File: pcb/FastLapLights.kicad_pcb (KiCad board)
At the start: 4 copper layers, 27.3 x 40 mm, 17 parts, among them J1 POWER_CON, J2 SWD, J3 PWR, J4 I2C, J5 Conn_02x04_Counter_Clockwise, U1 BD33FC0FP, U2 STM32C011F4Px

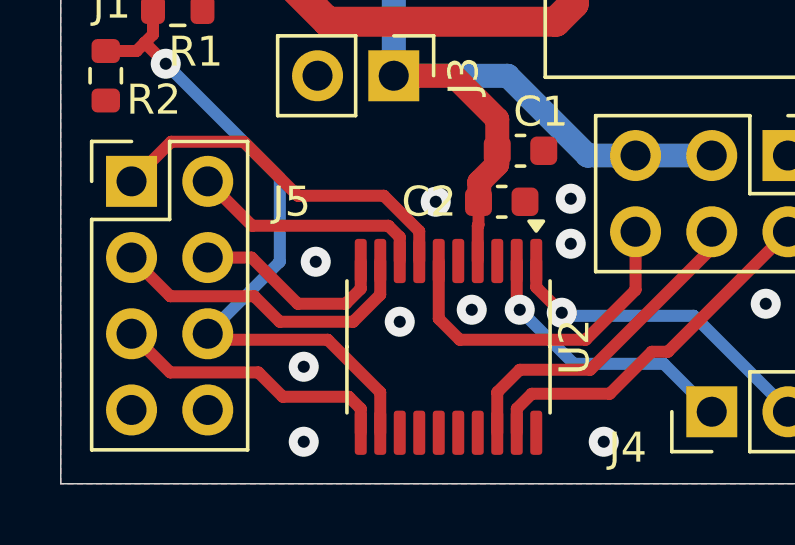
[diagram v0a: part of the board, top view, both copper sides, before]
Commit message: prep firmware
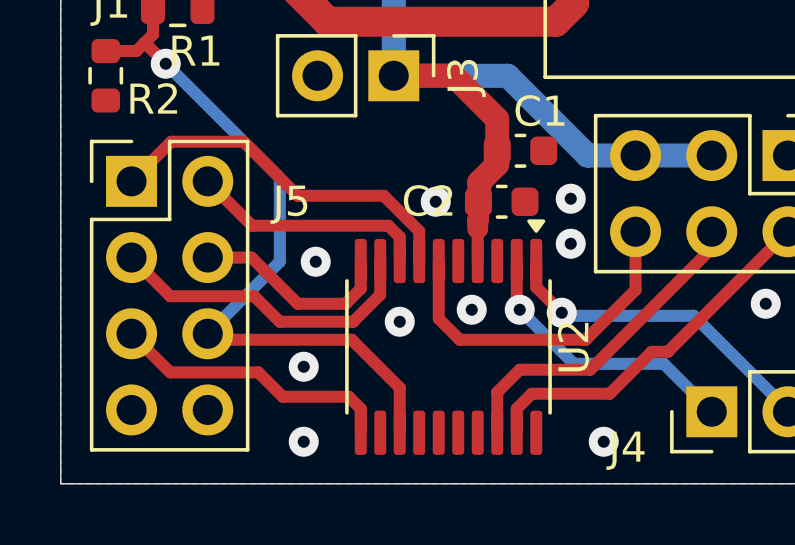
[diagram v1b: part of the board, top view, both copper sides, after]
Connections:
- U2 pad 12: /IO_POWER_RAIL_DATA -> unconnected-(U2-PA5-Pad12)
- U2 pad 13: unconnected-(U2-PA6-Pad13) -> /IO_POWER_RAIL_DATA
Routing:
- net /IO_POWER_RAIL_DATA: track 23.1 -> 23.8 mm
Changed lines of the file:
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@@
 	(net 13 "unconnected-(U2-PA9{slash}PA11-Pad16)")
 	(net 14 "unconnected-(U2-PC15-Pad3)")
-	(net 15 "unconnected-(U2-PA6-Pad13)")
+	(net 15 "unconnected-(U2-PA5-Pad12)")
 	(net 16 "unconnected-(U2-PA10{slash}PA12-Pad17)")
 	(net 17 "VRAIL")
@@
 			(layers "F.Cu" "F.Paste" "F.Mask")
 			(roundrect_rratio 0.25)
-			(net 18 "/IO_POWER_RAIL_DATA")
+			(net 15 "unconnected-(U2-PA5-Pad12)")
 			(pinfunction "PA5")
-			(pintype "bidirectional")
+			(pintype "bidirectional+no_connect")
 		)
 		(pad "13" smd roundrect
@@
 			(layers "F.Cu" "F.Paste" "F.Mask")
 			(roundrect_rratio 0.25)
-			(net 15 "unconnected-(U2-PA6-Pad13)")
+			(net 18 "/IO_POWER_RAIL_DATA")
 			(pinfunction "PA6")
-			(pintype "bidirectional+no_connect")
+			(pintype "bidirectional")
 		)
 		(pad "14" smd roundrect
@@
 		(layer "Cmts.User")
 		(pts
-			(xy 42.5 86.7) (xy 42.5 126.7)
+			(xy 42.5 86.7) (xy 42.5 103.6)
 		)
-		(height 7.799999)
-		(gr_text "40.0000 mm"
-			(at 32.900001 106.7 90)
+		(height 1.6)
+		(gr_text "16.9000 mm"
+			(at 39.75 95.15 90)
 			(layer "Cmts.User")
 			(effects
 				(font
-					(size 1.5 1.5)
-					(thickness 0.3)
+					(size 1 1)
+					(thickness 0.15)
 				)
 			)
@@
 		)
 		(style
-			(thickness 0.2)
+			(thickness 0.1)
 			(arrow_length 1.27)
 			(text_position_mode 0)
@@
 			(xy 42.5 126.7) (xy 69.8 126.7)
 		)
-		(height 8)
+		(height 10.7)
 		(gr_text "27.3000 mm"
-			(at 56.15 132.9 0)
+			(at 56.15 136.25 0)
+			(layer "Cmts.User")
+			(effects
+				(font
+					(size 1 1)
+					(thickness 0.15)
+				)
+			)
+		)
+		(format
+			(prefix "")
+			(suffix "")
+			(units 3)
+			(units_format 1)
+			(precision 4)
+		)
+		(style
+			(thickness 0.1)
+			(arrow_length 1.27)
+			(text_position_mode 0)
+			(extension_height 0.58642)
+			(extension_offset 0.5) keep_text_aligned)
+	)
+	(dimension
+		(type aligned)
+		(layer "Cmts.User")
+		(pts
+			(xy 42.5 86.7) (xy 42.5 114.9)
+		)
+		(height 6.9)
+		(gr_text "28.2000 mm"
+			(at 34.45 100.8 90)
 			(layer "Cmts.User")
 			(effects
 				(font
-					(size 1.5 1.5)
-					(thickness 0.3)
+					(size 1 1)
+					(thickness 0.15)
 				)
 			)
@@
 		)
 		(style
-			(thickness 0.2)
+			(thickness 0.1)
+			(arrow_length 1.27)
+			(text_position_mode 0)
+			(extension_height 0.58642)
+			(extension_offset 0.5) keep_text_aligned)
+	)
+	(dimension
+		(type aligned)
+		(layer "Cmts.User")
+		(pts
+			(xy 42.5 86.7) (xy 42.5 109.9)
+		)
+		(height 4.2)
+		(gr_text "23.2000 mm"
+			(at 37.15 98.3 90)
+			(layer "Cmts.User")
+			(effects
+				(font
+					(size 1 1)
+					(thickness 0.15)
+				)
+			)
+		)
+		(format
+			(prefix "")
+			(suffix "")
+			(units 3)
+			(units_format 1)
+			(precision 4)
+		)
+		(style
+			(thickness 0.1)
+			(arrow_length 1.27)
+			(text_position_mode 0)
+			(extension_height 0.58642)
+			(extension_offset 0.5) keep_text_aligned)
+	)
+	(dimension
+		(type aligned)
+		(layer "Cmts.User")
+		(pts
+			(xy 49.25 114.9) (xy 42.5 114.9)
+		)
+		(height -14.9)
+		(gr_text "6.75 mm"
+			(at 45.875 128.65 0)
+			(layer "Cmts.User")
+			(effects
+				(font
+					(size 1 1)
+					(thickness 0.15)
+				)
+			)
+		)
+		(format
+			(prefix "")
+			(suffix "")
+			(units 3)
+			(units_format 1)
+			(precision 2)
+		)
+		(style
+			(thickness 0.1)
+			(arrow_length 1.27)
+			(text_position_mode 0)
+			(extension_height 0.58642)
+			(extension_offset 0.5) keep_text_aligned)
+	)
+	(dimension
+		(type aligned)
+		(layer "Cmts.User")
+		(pts
+			(xy 55.4 114.9) (xy 42.5 114.9)
+		)
+		(height -17.8)
+		(gr_text "12.9000 mm"
+			(at 48.95 131.55 0)
+			(layer "Cmts.User")
+			(effects
+				(font
+					(size 1 1)
+					(thickness 0.15)
+				)
+			)
+		)
+		(format
+			(prefix "")
+			(suffix "")
+			(units 3)
+			(units_format 1)
+			(precision 4)
+		)
+		(style
+			(thickness 0.1)
+			(arrow_length 1.27)
+			(text_position_mode 0)
+			(extension_height 0.58642)
+			(extension_offset 0.5) keep_text_aligned)
+	)
+	(dimension
+		(type aligned)
+		(layer "Cmts.User")
+		(pts
+			(xy 42.5 86.7) (xy 42.5 126.7)
+		)
+		(height 9.9)
+		(gr_text "40.0000 mm"
+			(at 31.45 106.7 90)
+			(layer "Cmts.User")
+			(effects
+				(font
+					(size 1 1)
+					(thickness 0.15)
+				)
+			)
+		)
+		(format
+			(prefix "")
+			(suffix "")
+			(units 3)
+			(units_format 1)
+			(precision 4)
+		)
+		(style
+			(thickness 0.1)
 			(arrow_length 1.27)
 			(text_position_mode 0)
@@
 	)
 	(segment
+		(start 56.4 119.275)
+		(end 56.4 118.2)
+		(width 0.4)
+		(layer "F.Cu")
+		(net 3)
+	)
+	(segment
+		(start 56.4 117.9)
+		(end 56.425 117.875)
+		(width 0.7)
+		(layer "F.Cu")
+		(net 3)
+	)
+	(segment
 		(start 58.225 103.0275)
 		(end 58.2525 103)
@@
 	)
 	(segment
-		(start 56.4 118.1)
-		(end 56.425 118.075)
-		(width 0.4)
-		(layer "F.Cu")
-		(net 3)
-	)
-	(segment
 		(start 55.225 105.125)
 		(end 56.4 105.125)
@@
 	)
 	(segment
+		(start 56.425 117.875)
+		(end 56.425 117.3)
+		(width 0.7)
+		(layer "F.Cu")
+		(net 3)
+	)
+	(segment
 		(start 57.05 115.6)
 		(end 57.05 114.55)
@@
 	)
 	(segment
-		(start 56.4 119.275)
-		(end 56.4 118.1)
-		(width 0.4)
-		(layer "F.Cu")
-		(net 3)
-	)
-	(segment
 		(start 56.4 103.5)
 		(end 56.4 105.125)
@@
 	)
 	(segment
-		(start 57.05 115.6)
-		(end 57.05 116.05)
-		(width 0.8)
+		(start 56.4 118.2)
+		(end 56.4 117.9)
+		(width 0.7)
 		(layer "F.Cu")
 		(net 3)
 	)
 	(segment
-		(start 56.425 118.075)
-		(end 56.425 117.3)
-		(width 0.4)
+		(start 57.05 115.6)
+		(end 57.05 116.05)
+		(width 0.8)
 		(layer "F.Cu")
 		(net 3)
@@
 	)
 	(segment
-		(start 51.4 121.9)
-		(end 47.6 121.9)
+		(start 52.2 121.9)
+		(end 53.8 123.5)
 		(width 0.4)
 		(layer "F.Cu")
@@
 	)
 	(segment
-		(start 53.15 123.65)
-		(end 51.4 121.9)
+		(start 47.6 121.9)
+		(end 52.2 121.9)
 		(width 0.4)
 		(layer "F.Cu")
@@
 	)
 	(segment
-		(start 47.6 121.9)
-		(end 47.4 121.7)
+		(start 47.4 121.7)
+		(end 47.6 121.9)
 		(width 0.4)
 		(layer "F.Cu")
@@
 	)
 	(segment
-		(start 53.15 125)
-		(end 53.15 123.65)
+		(start 53.8 123.5)
+		(end 53.8 125)
 		(width 0.4)
 		(layer "F.Cu")
